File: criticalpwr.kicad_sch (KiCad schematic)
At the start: 2 parts, among them J3 Power Conn

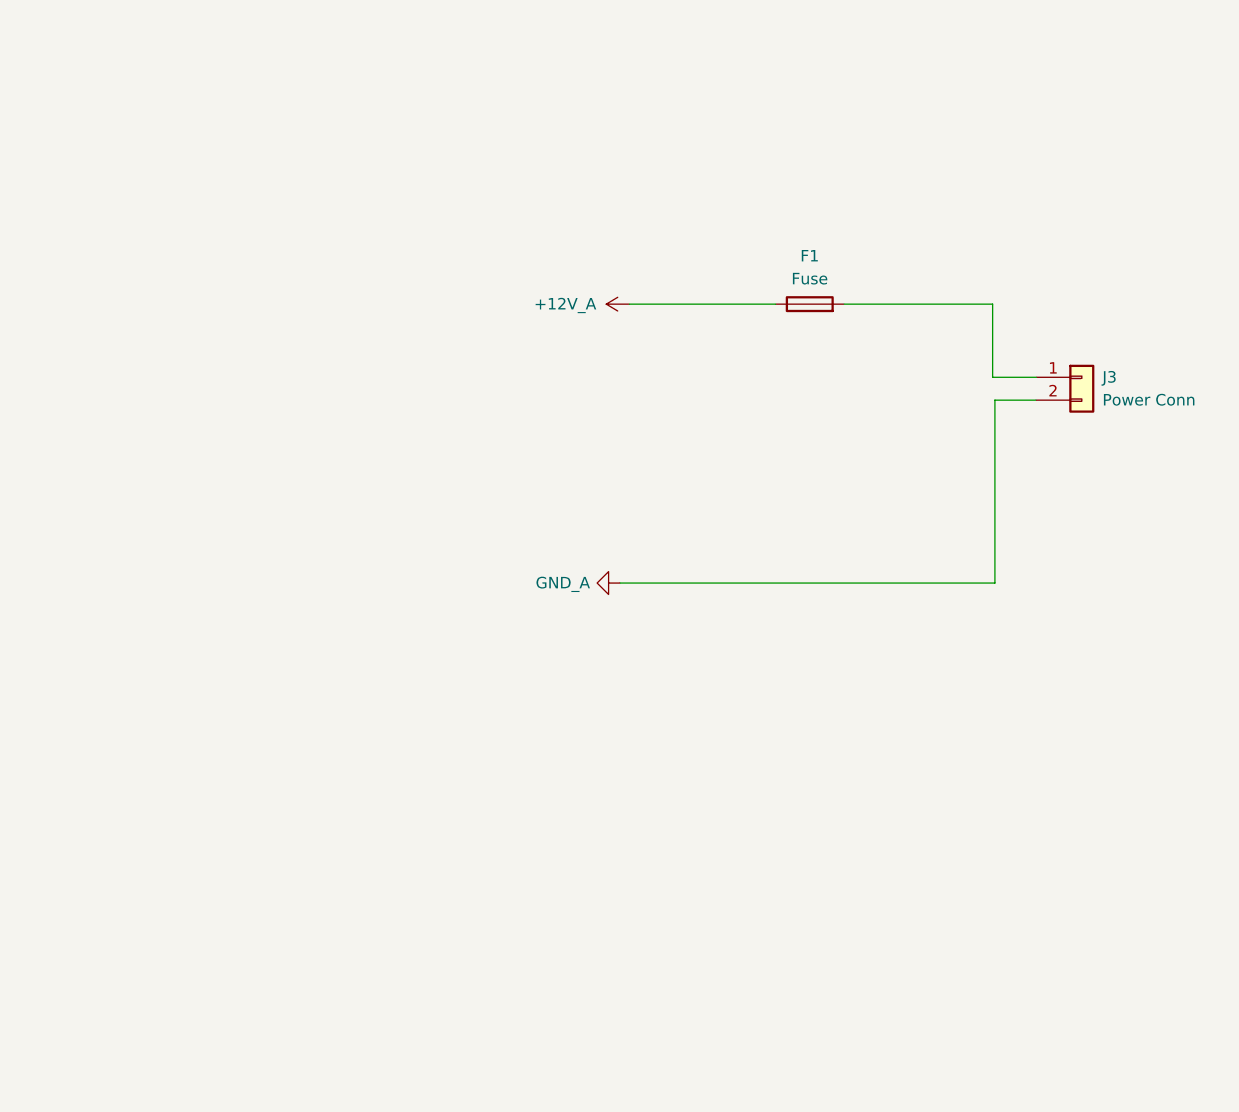
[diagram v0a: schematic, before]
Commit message: finished schematic
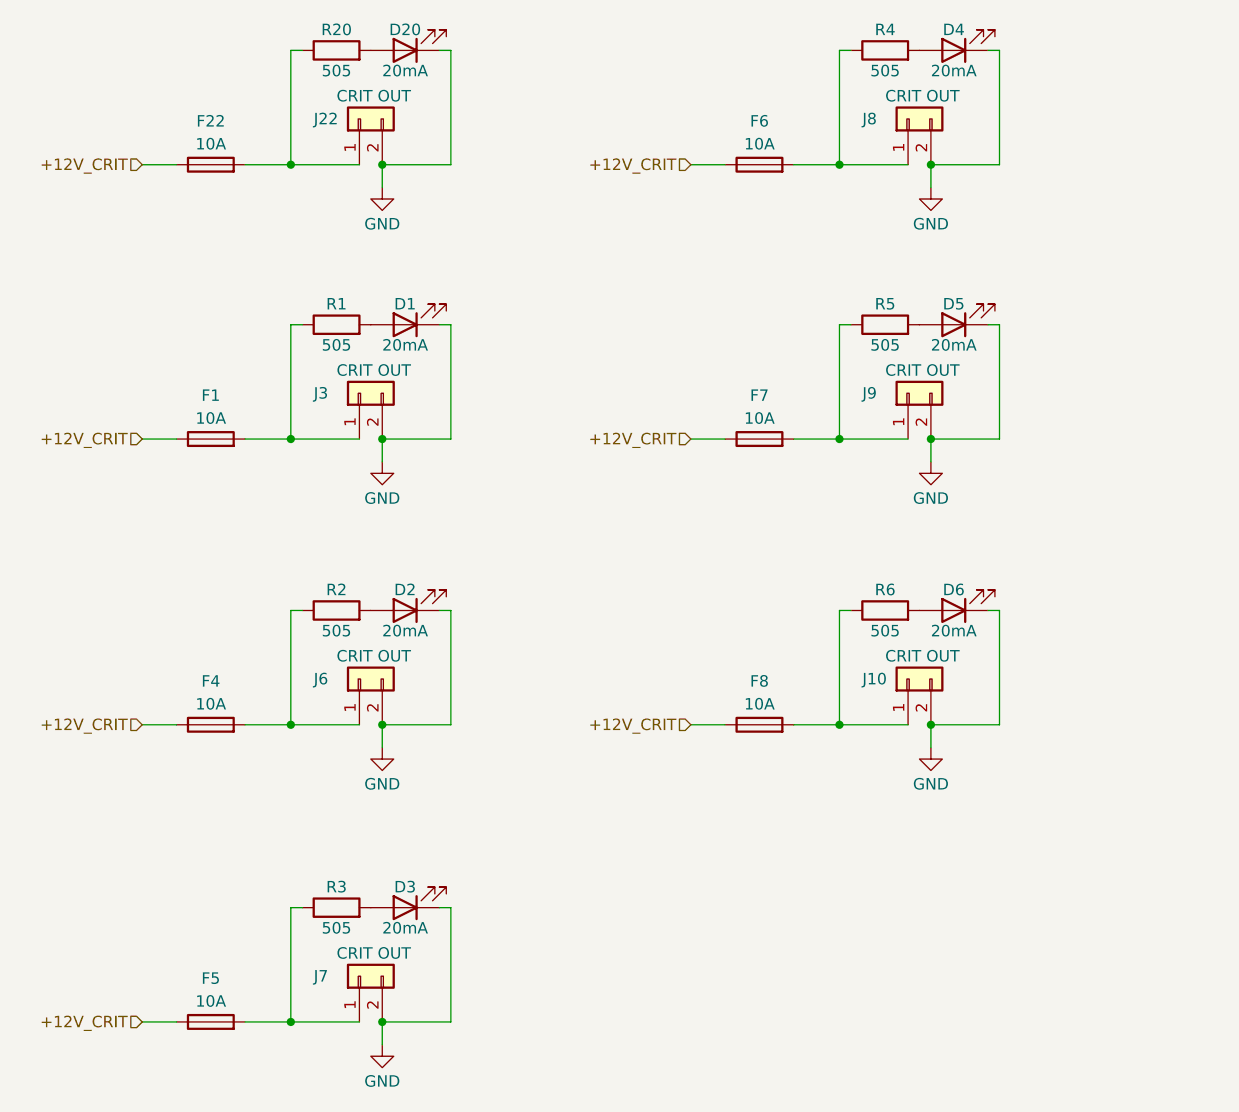
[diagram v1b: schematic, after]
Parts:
- added D1, D2, D20, D3, D4, D5, D6: 20mA, LED_SMD:LED_0805_2012Metric, symbol Device:LED
- added F22, F4, F5, F6, F7, F8: 10A, footprints:3588, symbol Device:Fuse
- added J10, J22, J6, J7, J8, J9: CRIT OUT, footprints:Molex_Micro-Fit_3.0_43650-0215_1x02_P3.00mm_Vertical, symbol Connector_Generic:Conn_01x02
- added R1, R2, R20, R3, R4, R5, R6: 505, Resistor_SMD:R_0805_2012Metric, symbol Device:R
- F1: value Fuse -> 10A
- J3: value Power Conn -> CRIT OUT
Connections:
- net at F1.2, J3.1 (Pin_1): now also R1.1
- net +12V_A renamed +12V_CRIT
- net +12V_CRIT: now also F22.1, F4.1, F5.1, F6.1, F7.1, F8.1
- net GND_A renamed GND
- net GND: now also D1.1 (K), D2.1 (K), D20.1 (K), D3.1 (K), D4.1 (K), D5.1 (K), D6.1 (K), J10.2 (Pin_2), J22.2 (Pin_2), J6.2 (Pin_2), J7.2 (Pin_2), J8.2 (Pin_2), J9.2 (Pin_2)
- new net: F5.2, J7.1 (Pin_1), R3.1
- new net: F4.2, J6.1 (Pin_1), R2.1
- new net: D6.2 (A), R6.2
- new net: F22.2, J22.1 (Pin_1), R20.1
- new net: D20.2 (A), R20.2
- new net: D1.2 (A), R1.2
- new net: F8.2, J10.1 (Pin_1), R6.1
- new net: D2.2 (A), R2.2
- new net: D4.2 (A), R4.2
- new net: F6.2, J8.1 (Pin_1), R4.1
- new net: F7.2, J9.1 (Pin_1), R5.1
- new net: D5.2 (A), R5.2
- new net: D3.2 (A), R3.2
